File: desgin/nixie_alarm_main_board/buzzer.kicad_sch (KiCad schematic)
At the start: 1 part

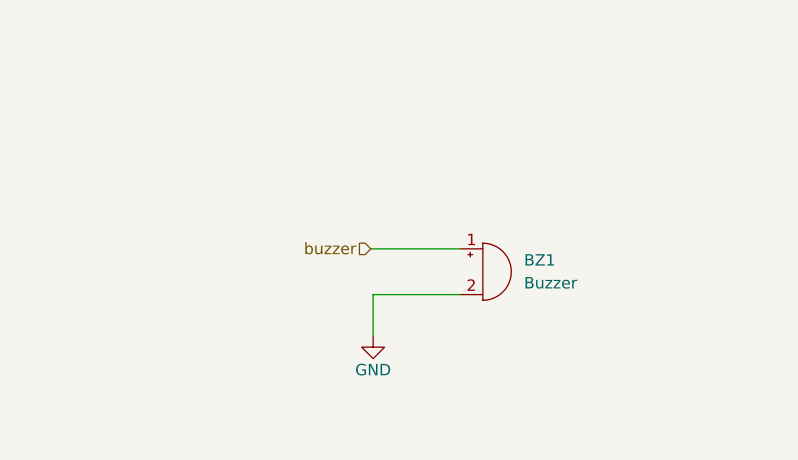
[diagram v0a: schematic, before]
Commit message: filter caps
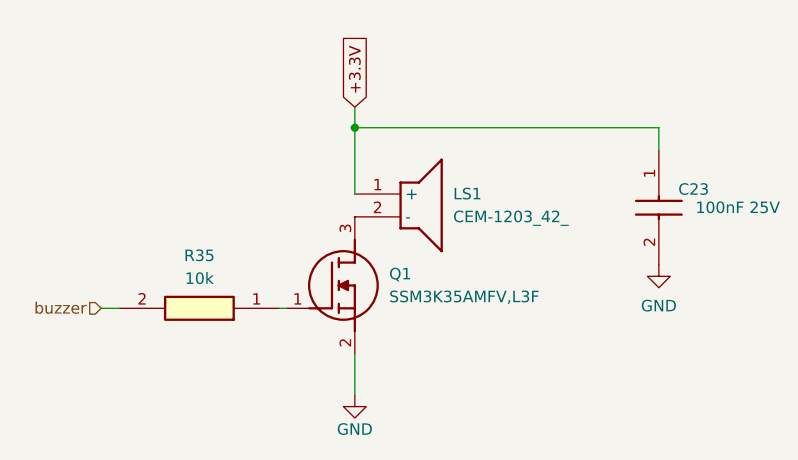
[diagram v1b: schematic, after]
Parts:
- removed BZ1: Buzzer, Buzzer_Beeper:MagneticBuzzer_PUI_AT-0927-TT-6-R, symbol Device:Buzzer
- added C23: 100nF 25V, GRM033D70J224ME01D, symbol SamacSys_Parts:GRM033R71E101KA01J
- added LS1: CEM-1203_42_, SamacSys_Parts:CEM-1203_42_, symbol SamacSys_Parts:CEM-1203_42_
- added Q1: SSM3K35AMFV,L3F, SSM3K35AMFVL3F, symbol SamacSys_Parts:SSM3K35AMFV,L3F
- added R35: 10k, ERJUP6, symbol SamacSys_Parts:ERJ-UP6D5101V
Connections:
- net GND: now also C23.2, Q1.2 (S)
- net buzzer: now also R35.2
- new net: LS1.2 (-), Q1.3 (D)
- new net: Q1.1 (G), R35.1
- new net +3.3V: C23.1, LS1.1 (+)

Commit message: new caps footprint
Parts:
- C23: footprint GRM033D70J224ME01D -> Capacitor_SMD:C_0805_2012Metric_Pad1.18x1.45mm_HandSolder
- R35: footprint ERJUP6 -> Resistor_SMD:R_0805_2012Metric_Pad1.20x1.40mm_HandSolder
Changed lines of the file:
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@@
 			)
 		)
-		(property "Footprint" "GRM033D70J224ME01D"
+		(property "Footprint" "Capacitor_SMD:C_0805_2012Metric_Pad1.18x1.45mm_HandSolder"
 			(at 82.88 87.63 0)
 			(effects
@@
 			)
 		)
-		(property "Footprint" "ERJUP6"
+		(property "Footprint" "Resistor_SMD:R_0805_2012Metric_Pad1.20x1.40mm_HandSolder"
 			(at 122.936 0.076 0)
 			(effects
